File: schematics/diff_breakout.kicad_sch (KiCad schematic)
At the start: 24 parts, among them J1 Conn_01x06_Pin, J2 Conn_01x06_Pin, J3 Conn_01x06_Pin, J4 Conn_01x06_Pin, J5 Conn_01x06_Pin, J6 Conn_01x06_Pin, J7 Screw_Terminal_01x02, U6 LM2596S-3.3, U8 AP2112K-3.3TRG1

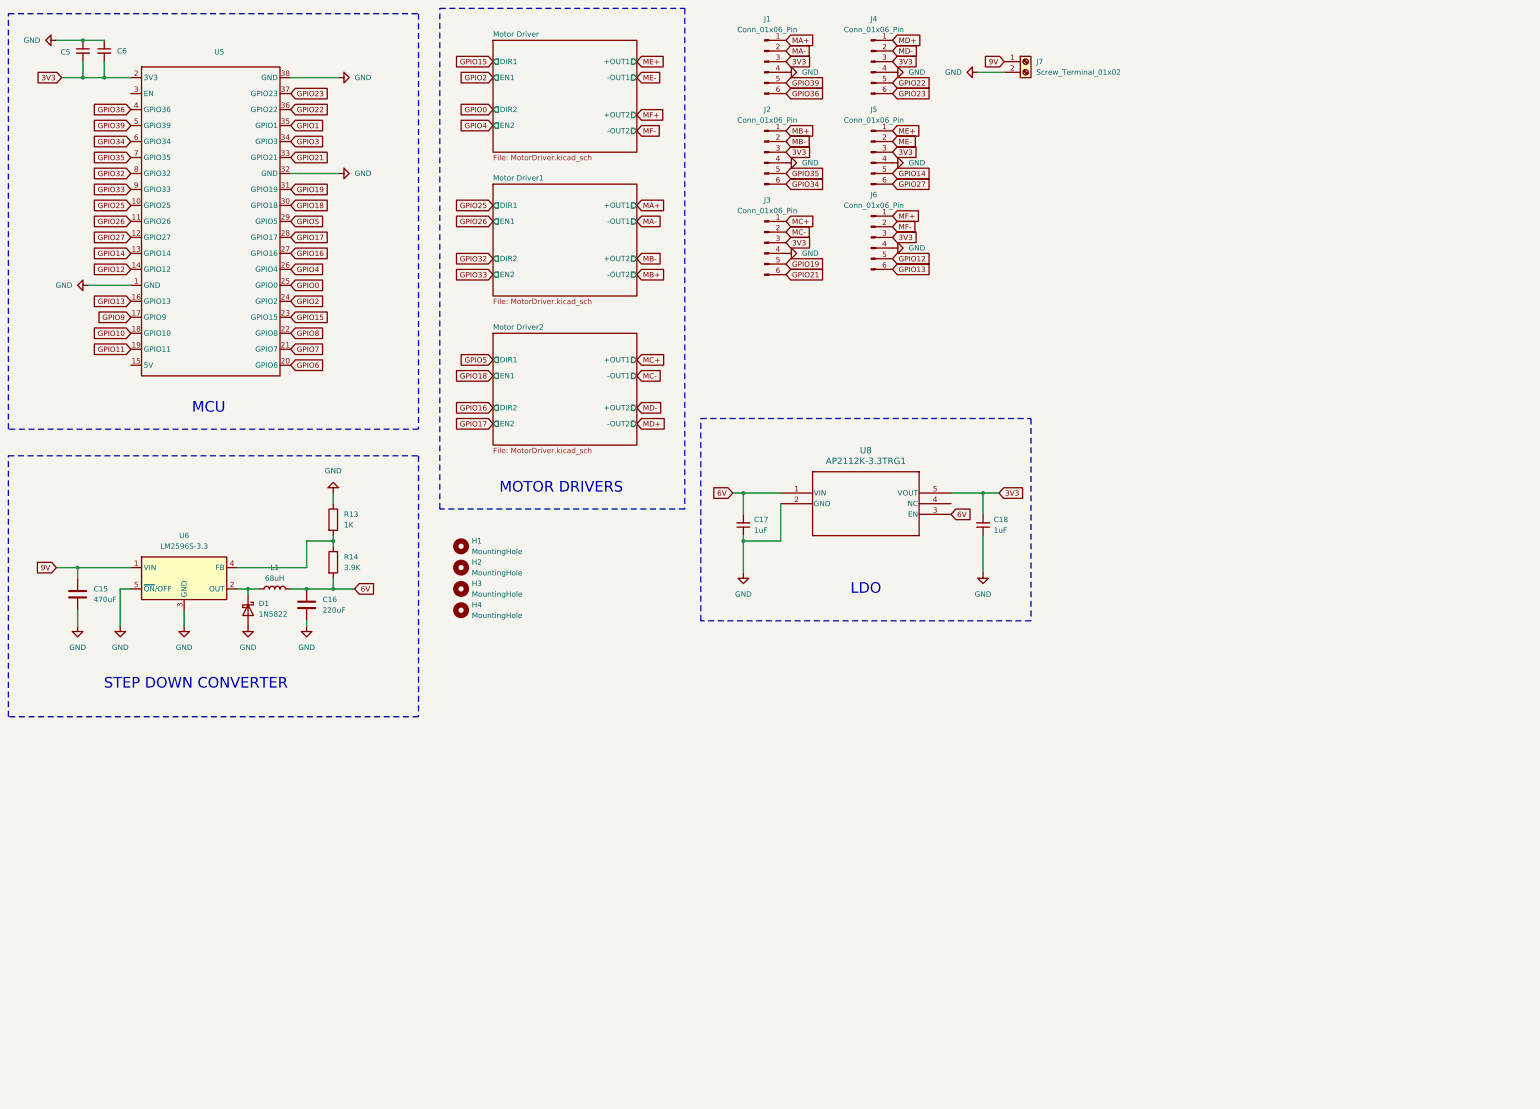
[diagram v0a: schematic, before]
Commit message: changed one of the schematics
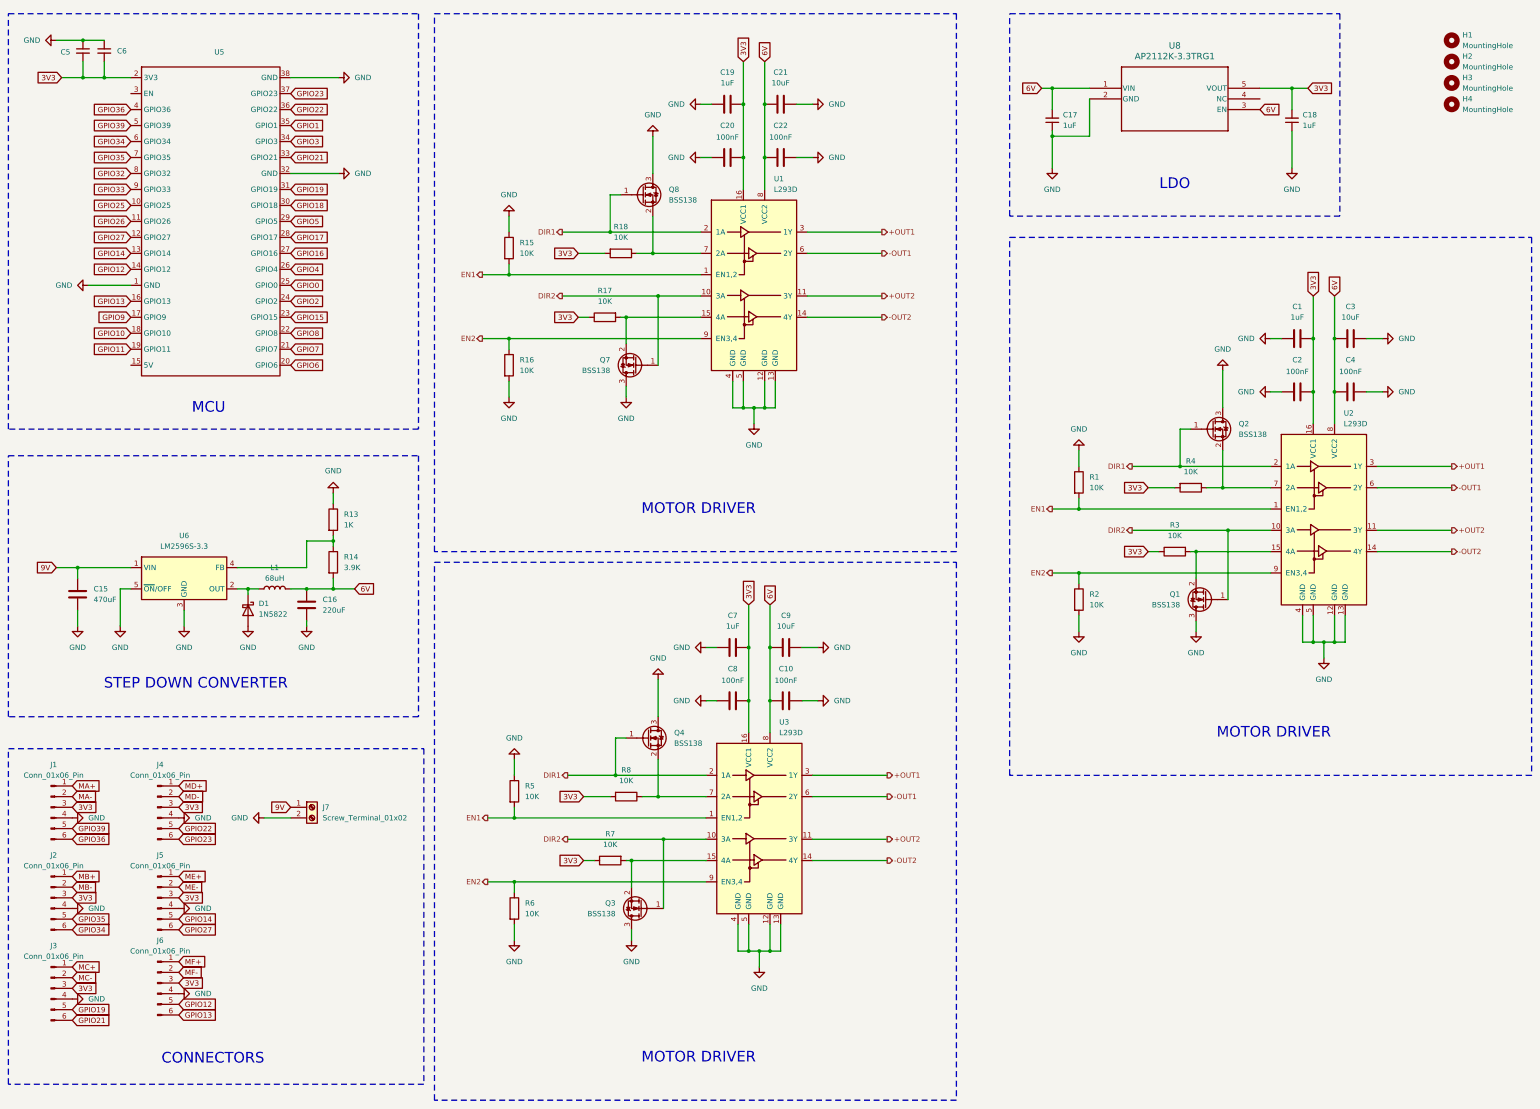
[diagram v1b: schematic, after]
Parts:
- added C1, C19, C7: 1uF, Capacitor_SMD:C_1210_3225Metric, symbol Device:C
- added C10, C2, C20, C22, C4, C8: 100nF, Capacitor_SMD:C_0805_2012Metric, symbol Device:C
- added C21, C3, C9: 10uF, Capacitor_SMD:C_1210_3225Metric, symbol Device:C
- added Q1, Q2, Q3, Q4, Q7, Q8: BSS138, Package_TO_SOT_SMD:SOT-23, symbol Transistor_FET:BSS138
- added R1, R15, R16, R17, R18, R2, R3, R4, R5, R6, R7, R8: 10K, Resistor_SMD:R_0603_1608Metric, symbol Device:R
- added U1, U2, U3: L293D, Package_DIP:DIP-16_W7.62mm, symbol Driver_Motor:L293D
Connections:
- net 3V3: now also C1.2, C19.2, C2.1, C20.1, C7.2, C8.1, R17.1, R18.2, R3.1, R4.2, R7.1, R8.2, U1.16 (VCC1), U2.16 (VCC1), U3.16 (VCC1)
- net 6V: now also C10.2, C21.1, C22.2, C3.1, C4.2, C9.1, U1.8 (VCC2), U2.8 (VCC2), U3.8 (VCC2)
- net GND: now also C1.1, C10.1, C19.1, C2.2, C20.2, C21.2, C22.1, C3.2, C4.1, C7.1, C8.2, C9.2, Q1.3 (D), Q2.3 (D), Q3.3 (D), Q4.3 (D), Q7.3 (D), Q8.3 (D), R1.1, R15.1, R16.2, R2.2, R5.1, R6.2, U1.12 (GND), U1.13 (GND), U1.4 (GND), U1.5 (GND), U2.12 (GND), U2.13 (GND), U2.4 (GND), U2.5 (GND), U3.12 (GND), U3.13 (GND), U3.4 (GND), U3.5 (GND)
- new net: Q8.2 (S), R18.1, U1.7 (2A)
- new net: Q3.2 (S), R7.2, U3.15 (4A)
- new net: Q4.2 (S), R8.1, U3.7 (2A)
- new net: Q2.2 (S), R4.1, U2.7 (2A)
- new net: Q1.2 (S), R3.2, U2.15 (4A)
- new net: Q7.2 (S), R17.2, U1.15 (4A)
- new net +OUT1: U1.3 (1Y), U2.3 (1Y), U3.3 (1Y)
- new net +OUT2: U1.11 (3Y), U2.11 (3Y), U3.11 (3Y)
- new net -OUT1: U1.6 (2Y), U2.6 (2Y), U3.6 (2Y)
- new net -OUT2: U1.14 (4Y), U2.14 (4Y), U3.14 (4Y)
- new net DIR1: Q2.1 (G), Q4.1 (G), Q8.1 (G), U1.2 (1A), U2.2 (1A), U3.2 (1A)
- new net DIR2: Q1.1 (G), Q3.1 (G), Q7.1 (G), U1.10 (3A), U2.10 (3A), U3.10 (3A)
- new net EN1: R1.2, R15.2, R5.2, U1.1 (EN1,2), U2.1 (EN1,2), U3.1 (EN1,2)
- new net EN2: R16.1, R2.1, R6.1, U1.9 (EN3,4), U2.9 (EN3,4), U3.9 (EN3,4)
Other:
- removed sheet Motor Driver
- removed sheet Motor Driver1
- removed sheet Motor Driver2
- note added: "CONNECTORS"
- note added: "MOTOR DRIVER"
- note removed: "MOTOR DRIVERS"
- moved on the sheet: C17, C18, H1, H2, H3, H4, J1, J2, J3, J4, J5, J6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
